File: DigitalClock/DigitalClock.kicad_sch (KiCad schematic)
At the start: 46 parts, among them J1 Battery, Q1 2N3904, Q2 2N3904, Q3 2N3904, SW1 +HOUR, SW2 SET TIME, SW3 +MIN, U1 74LS47, U10 HDSP-7801, U11 LM1117-5.0, U12 74LS47, U13 74LS74, U14 HDSP-7801, U15 74LS04, U2 NE555P, U3 HDSP-7801, U4 74LS08, U5 74LS32, U6 74LS47, U7 HDSP-7801, U8 74LS47, U9 74LS74

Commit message: about to begin layout
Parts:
- C1, C2, C3, C4: footprint (none) -> Capacitor_THT:C_Disc_D5.0mm_W2.5mm_P5.00mm
- C5, C6, C7: footprint (none) -> Capacitor_THT:CP_Radial_Tantal_D5.0mm_P5.00mm
- D1, D2: footprint (none) -> LED_THT:LED_D3.0mm
- J1: footprint (none) -> TerminalBlock_Phoenix:TerminalBlock_Phoenix_MKDS-1,5-2_1x02_P5.00mm_Horizontal
- R1, R10, R11, R12, R13, R14, R15, R2, R3, R4, R5, R6, R7, R8, R9: footprint (none) -> Resistor_THT:R_Axial_DIN0207_L6.3mm_D2.5mm_P10.16mm_Horizontal
- SW1, SW2, SW3: footprint (none) -> Button_Switch_THT:Push_E-Switch_KS01Q01
- U1, U12, U6, U8: footprint (none) -> Package_DIP:DIP-16_W7.62mm
- U10, U14, U3, U7: footprint Display_7Segment:HDSP-7801 -> Display_7Segment:7SegmentLED_LTS6760_LTS6780
- U11: footprint (none) -> Package_TO_SOT_THT:TO-220-3_Vertical
- U13, U15, U4, U5, U9: footprint (none) -> Package_DIP:DIP-14_W7.62mm

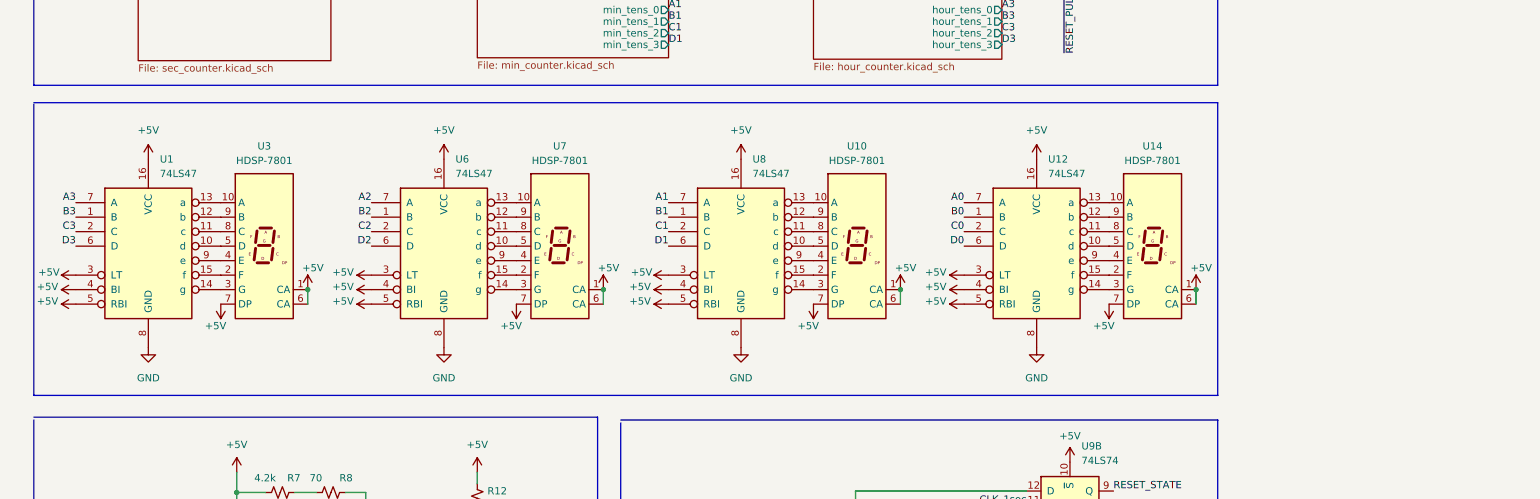
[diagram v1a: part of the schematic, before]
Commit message: more routing
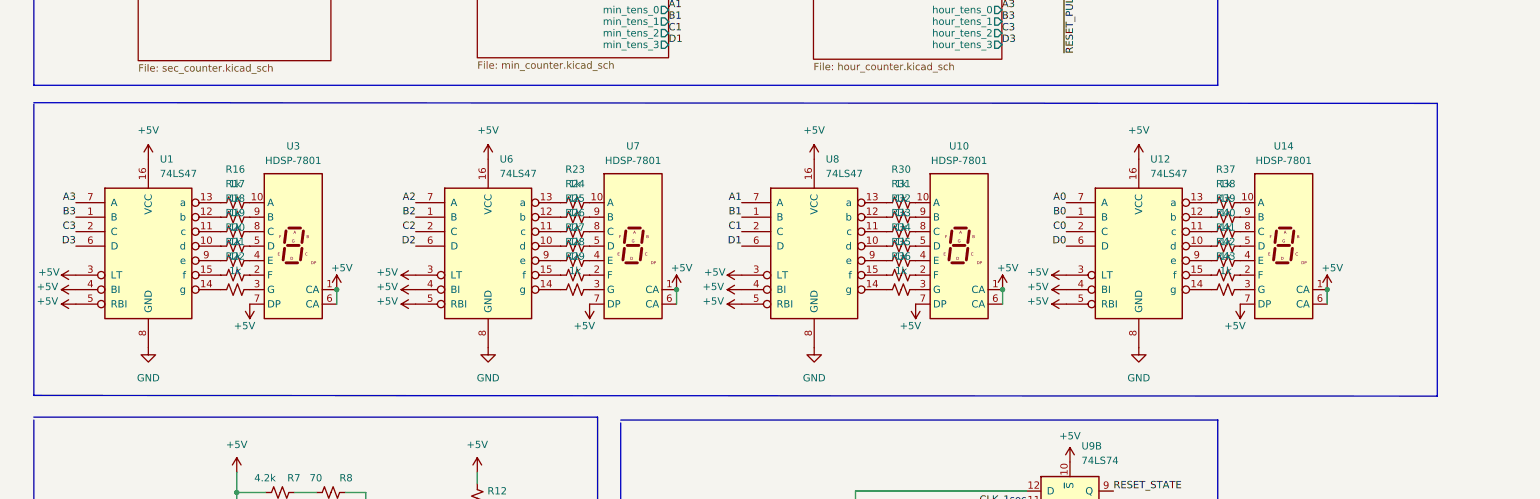
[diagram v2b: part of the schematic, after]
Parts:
- added R16, R17, R18, R19, R20, R21, R22, R23, R24, R25, R26, R27, R28, R29, R30, R31, R32, R33, R34, R35, R36, R37, R38, R39, R40, R41, R42, R43: 1k, Resistor_THT:R_Axial_DIN0207_L6.3mm_D2.5mm_P10.16mm_Horizontal, symbol Device:R_Small_US
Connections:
- net at U7.10 (A): now also R23.2; no longer U6.13 (a)
- net at U7.2 (F): now also R28.2; no longer U6.15 (f)
- net at U7.3 (G): now also R29.2; no longer U6.14 (g)
- net at U7.4 (E): now also R27.2; no longer U6.9 (e)
- net at U7.5 (D): now also R26.2; no longer U6.10 (d)
- net at U7.8 (C): now also R25.2; no longer U6.11 (c)
- net at U7.9 (B): now also R24.2; no longer U6.12 (b)
- net at U1.10 (d): now also R19.1; no longer U3.5 (D)
- net at U1.11 (c): now also R18.1; no longer U3.8 (C)
- net at U1.12 (b): now also R17.1; no longer U3.9 (B)
- net at U1.13 (a): now also R16.1; no longer U3.10 (A)
- net at U1.14 (g): now also R22.1; no longer U3.3 (G)
- net at U1.15 (f): now also R21.1; no longer U3.2 (F)
- net at U1.9 (e): now also R20.1; no longer U3.4 (E)
- net at U8.13 (a): now also R30.1; no longer U10.10 (A)
- net at U10.2 (F): now also R35.2; no longer U8.15 (f)
- net at U8.14 (g): now also R36.1; no longer U10.3 (G)
- net at U10.4 (E): now also R34.2; no longer U8.9 (e)
- net at U8.10 (d): now also R33.1; no longer U10.5 (D)
- net at U10.8 (C): now also R32.2; no longer U8.11 (c)
- net at U10.9 (B): now also R31.2; no longer U8.12 (b)
- net at U14.10 (A): now also R37.2; no longer U12.13 (a)
- net at U14.2 (F): now also R42.2; no longer U12.15 (f)
- net at U12.14 (g): now also R43.1; no longer U14.3 (G)
- net at U12.9 (e): now also R41.1; no longer U14.4 (E)
- net at U14.5 (D): now also R40.2; no longer U12.10 (d)
- net at U14.8 (C): now also R39.2; no longer U12.11 (c)
- net at U12.12 (b): now also R38.1; no longer U14.9 (B)
- new net: R43.2, U14.3 (G)
- new net: R41.2, U14.4 (E)
- new net: R36.2, U10.3 (G)
- new net: R22.2, U3.3 (G)
- new net: R30.2, U10.10 (A)
- new net: R33.2, U10.5 (D)
- new net: R23.1, U6.13 (a)
- new net: R38.2, U14.9 (B)
- new net: R29.1, U6.14 (g)
- new net: R25.1, U6.11 (c)
- new net: R32.1, U8.11 (c)
- new net: R31.1, U8.12 (b)
- new net: R35.1, U8.15 (f)
- new net: R34.1, U8.9 (e)
- new net: R27.1, U6.9 (e)
- new net: R26.1, U6.10 (d)
- new net: R28.1, U6.15 (f)
- new net: R40.1, U12.10 (d)
- new net: R39.1, U12.11 (c)
- new net: R37.1, U12.13 (a)
- new net: R42.1, U12.15 (f)
- new net: R18.2, U3.8 (C)
- new net: R24.1, U6.12 (b)
- new net: R17.2, U3.9 (B)
- new net: R20.2, U3.4 (E)
- new net: R16.2, U3.10 (A)
- new net: R21.2, U3.2 (F)
- new net: R19.2, U3.5 (D)
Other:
- moved on the sheet: U10, U12, U14, U3, U6, U7, U8
